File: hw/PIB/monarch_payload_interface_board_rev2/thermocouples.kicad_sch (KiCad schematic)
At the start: 30 parts, among them U3 MAX31856MUD_T, U5 MAX31856MUD_T, U6 MAX31856MUD_T, U7 MAX31856MUD_T, U8 MAX31856MUD_T

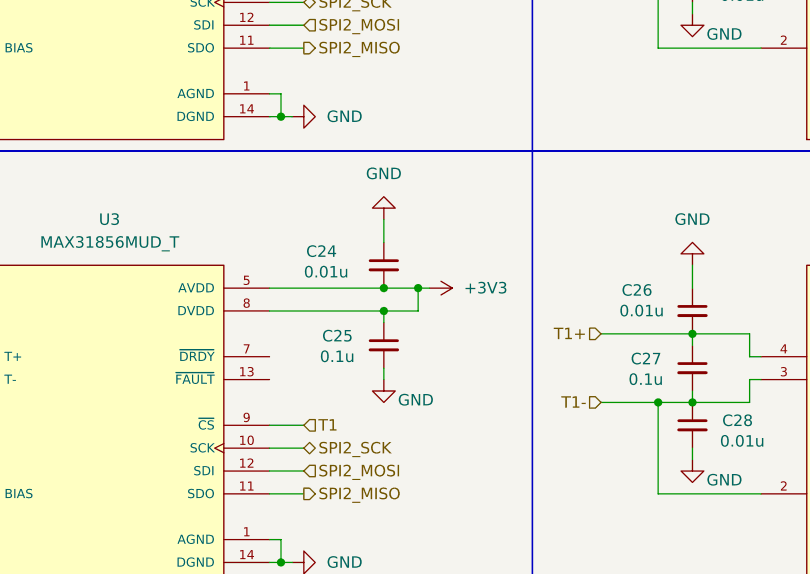
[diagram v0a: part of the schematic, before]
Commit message: AD7124 Fixes
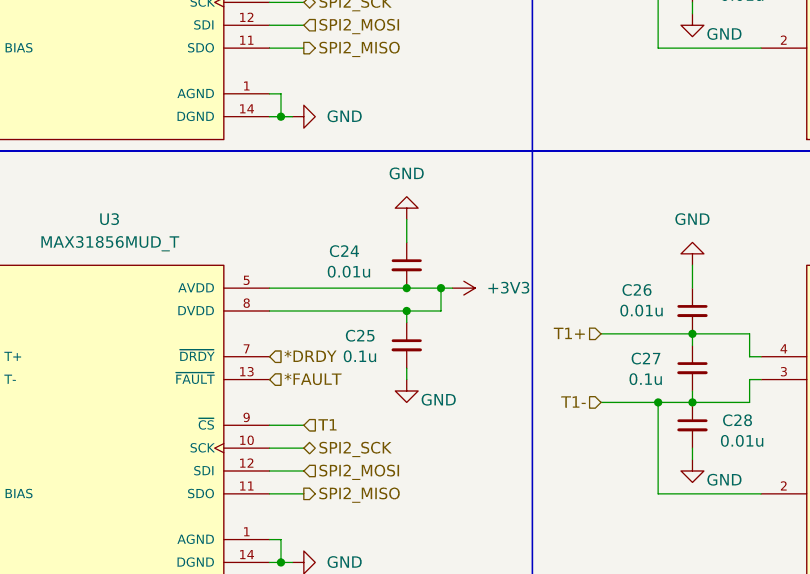
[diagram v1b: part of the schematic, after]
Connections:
- net *FAULT: now reaches U3.13 (~{FAULT})
- net *DRDY: now reaches U3.7 (~{DRDY})
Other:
- moved on the sheet: C24, C25
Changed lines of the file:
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@@
 	)
 	(junction
-		(at 86.36 78.74)
-		(diameter 0)
-		(color 0 0 0 0)
-	)
-	(junction
-		(at 86.36 81.28)
+		(at 88.9 81.28)
 		(diameter 0)
 		(color 0 0 0 0)
@@
 	)
 	(junction
-		(at 90.17 78.74)
+		(at 92.71 78.74)
 		(diameter 0)
 		(color 0 0 0 0)
@@
 	)
 	(junction
+		(at 88.9 78.74)
+		(diameter 0)
+		(color 0 0 0 0)
+	)
+	(junction
 		(at 210.82 34.29)
 		(diameter 0)
@@
 	(wire
 		(pts
-			(xy 86.36 82.55) (xy 86.36 81.28)
+			(xy 88.9 82.55) (xy 88.9 81.28)
 		)
 		(stroke
@@
 	(wire
 		(pts
-			(xy 90.17 78.74) (xy 91.44 78.74)
-		)
-		(stroke
-			(width 0)
-			(type default)
-		)
-	)
-	(wire
-		(pts
 			(xy 128.27 88.9) (xy 127 88.9)
 		)
@@
 	(wire
 		(pts
+			(xy 73.66 78.74) (xy 88.9 78.74)
+		)
+		(stroke
+			(width 0)
+			(type default)
+		)
+	)
+	(wire
+		(pts
 			(xy 110.49 41.91) (xy 116.84 41.91)
 		)
@@
 	(wire
 		(pts
-			(xy 86.36 88.9) (xy 86.36 87.63)
+			(xy 88.9 88.9) (xy 88.9 87.63)
 		)
 		(stroke
@@
 	(wire
 		(pts
-			(xy 73.66 78.74) (xy 86.36 78.74)
+			(xy 38.1 36.83) (xy 36.83 36.83)
 		)
 		(stroke
@@
 	(wire
 		(pts
-			(xy 38.1 36.83) (xy 36.83 36.83)
+			(xy 73.66 96.52) (xy 77.47 96.52)
 		)
 		(stroke
@@
 	(wire
 		(pts
-			(xy 73.66 96.52) (xy 77.47 96.52)
+			(xy 38.1 39.37) (xy 36.83 39.37)
 		)
 		(stroke
@@
 	(wire
 		(pts
-			(xy 38.1 39.37) (xy 36.83 39.37)
+			(xy 207.01 52.07) (xy 207.01 41.91)
 		)
 		(stroke
@@
 	(wire
 		(pts
-			(xy 207.01 52.07) (xy 207.01 41.91)
+			(xy 20.32 91.44) (xy 26.67 91.44)
 		)
 		(stroke
@@
 	(wire
 		(pts
-			(xy 20.32 91.44) (xy 26.67 91.44)
+			(xy 128.27 86.36) (xy 127 86.36)
 		)
 		(stroke
@@
 	(wire
 		(pts
-			(xy 128.27 86.36) (xy 127 86.36)
+			(xy 73.66 81.28) (xy 88.9 81.28)
 		)
 		(stroke
@@
 	(wire
 		(pts
-			(xy 86.36 71.12) (xy 86.36 73.66)
+			(xy 88.9 71.12) (xy 88.9 73.66)
 		)
 		(stroke
@@
 	(wire
 		(pts
-			(xy 90.17 78.74) (xy 90.17 81.28)
+			(xy 92.71 78.74) (xy 92.71 81.28)
 		)
 		(stroke
@@
 	(wire
 		(pts
-			(xy 73.66 81.28) (xy 86.36 81.28)
-		)
-		(stroke
-			(width 0)
-			(type default)
-		)
-	)
-	(wire
-		(pts
-			(xy 86.36 78.74) (xy 90.17 78.74)
+			(xy 88.9 78.74) (xy 93.98 78.74)
 		)
 		(stroke
@@
 	(wire
 		(pts
-			(xy 90.17 81.28) (xy 86.36 81.28)
+			(xy 92.71 81.28) (xy 88.9 81.28)
 		)
 		(stroke
@@
 		)
 	)
+	(hierarchical_label "*FAULT"
+		(shape input)
+		(at 73.66 88.9 0)
+		(effects
+			(font
+				(size 1.27 1.27)
+			)
+			(justify left)
+		)
+	)
 	(hierarchical_label "SPI2_MOSI"
 		(shape input)
@@
 		)
 	)
+	(hierarchical_label "*DRDY"
+		(shape input)
+		(at 73.66 86.36 0)
+		(effects
+			(font
+				(size 1.27 1.27)
+			)
+			(justify left)
+		)
+	)
 	(symbol
 		(lib_id "power:GND")
@@
 	(symbol
 		(lib_id "power:GND")
-		(at 86.36 71.12 180)
+		(at 88.9 71.12 180)
 		(unit 1)
 		(body_style 1)
@@
 		(fields_autoplaced yes)
 		(property "Reference" "#PWR047"
-			(at 86.36 64.77 0)
+			(at 88.9 64.77 0)
 			(hide yes)
 			(show_name no)
@@
 		)
 		(property "Value" "GND"
-			(at 86.36 66.04 0)
+			(at 88.9 66.04 0)
 			(show_name no)
 			(do_not_autoplace no)
@@
 		)
 		(property "Footprint" ""
-			(at 86.36 71.12 0)
+			(at 88.9 71.12 0)
 			(hide yes)
 			(show_name no)
@@
 		)
 		(property "Datasheet" ""
-			(at 86.36 71.12 0)
+			(at 88.9 71.12 0)
 			(hide yes)
 			(show_name no)
@@
 		)
 		(property "Description" "Power symbol creates a global label with name \"GND\" , ground"
-			(at 86.36 71.12 0)
+			(at 88.9 71.12 0)
 			(hide yes)
 			(show_name no)
@@
 	(symbol
 		(lib_id "Device:C_Small")
-		(at 86.36 85.09 0)
+		(at 88.9 85.09 0)
 		(unit 1)
 		(body_style 1)
@@
 		(dnp no)
 		(property "Reference" "C25"
-			(at 79.502 84.074 0)
+			(at 82.042 84.074 0)
 			(show_name no)
 			(do_not_autoplace no)
@@
 		)
 		(property "Value" "0.1u"
-			(at 79.248 86.36 0)
+			(at 81.788 86.36 0)
 			(show_name no)
 			(do_not_autoplace no)
@@
 		)
 		(property "Footprint" "Capacitor_SMD:C_0603_1608Metric"
-			(at 86.36 85.09 0)
+			(at 88.9 85.09 0)
 			(hide yes)
 			(show_name no)
@@
 		)
 		(property "Datasheet" ""
-			(at 86.36 85.09 0)
+			(at 88.9 85.09 0)
 			(hide yes)
 			(show_name no)
@@
 		)
 		(property "Description" "Unpolarized capacitor, small symbol"
-			(at 86.36 85.09 0)
+			(at 88.9 85.09 0)
 			(hide yes)
 			(show_name no)
@@
 	(symbol
 		(lib_id "power:GND")
-		(at 86.36 88.9 0)
+		(at 88.9 88.9 0)
 		(unit 1)
 		(body_style 1)
@@
 		(dnp no)
 		(property "Reference" "#PWR048"
-			(at 86.36 95.25 0)
+			(at 88.9 95.25 0)
 			(hide yes)
 			(show_name no)
@@
 		)
 		(property "Value" "GND"
-			(at 89.916 91.186 0)
+			(at 92.456 91.186 0)
 			(show_name no)
 			(do_not_autoplace no)
@@
 		)
 		(property "Footprint" ""
-			(at 86.36 88.9 0)
+			(at 88.9 88.9 0)
 			(hide yes)
 			(show_name no)
@@
 		)
 		(property "Datasheet" ""
-			(at 86.36 88.9 0)
+			(at 88.9 88.9 0)
 			(hide yes)
 			(show_name no)
@@
 		)
 		(property "Description" "Power symbol creates a global label with name \"GND\" , ground"
-			(at 86.36 88.9 0)
+			(at 88.9 88.9 0)
 			(hide yes)
 			(show_name no)
@@
 	(symbol
 		(lib_id "power:+3V3")
-		(at 91.44 78.74 270)
+		(at 93.98 78.74 270)
 		(unit 1)
 		(body_style 1)
@@
 		(fields_autoplaced yes)
 		(property "Reference" "#PWR046"
-			(at 87.63 78.74 0)
+			(at 90.17 78.74 0)
 			(hide yes)
 			(show_name no)
@@
 		)
 		(property "Value" "+3V3"
-			(at 95.25 78.7399 90)
+			(at 97.79 78.7399 90)
 			(show_name no)
 			(do_not_autoplace no)
@@
 		)
 		(property "Footprint" ""
-			(at 91.44 78.74 0)
+			(at 93.98 78.74 0)
 			(hide yes)
 			(show_name no)
@@
 		)
 		(property "Datasheet" ""
-			(at 91.44 78.74 0)
+			(at 93.98 78.74 0)
 			(hide yes)
 			(show_name no)
@@
 		)
 		(property "Description" "Power symbol creates a global label with name \"+3V3\""
-			(at 91.44 78.74 0)
+			(at 93.98 78.74 0)
 			(hide yes)
 			(show_name no)
@@
 	(symbol
 		(lib_id "Device:C_Small")
-		(at 86.36 76.2 0)
+		(at 88.9 76.2 0)
 		(unit 1)
 		(body_style 1)
@@
 		(dnp no)
 		(property "Reference" "C24"
-			(at 77.724 74.676 0)
+			(at 80.264 74.676 0)
 			(show_name no)
 			(do_not_autoplace no)
@@
 		)
 		(property "Value" "0.01u"
-			(at 77.47 76.962 0)
+			(at 80.01 76.962 0)
 			(show_name no)
 			(do_not_autoplace no)
@@
 		)
 		(property "Footprint" "Capacitor_SMD:C_0603_1608Metric"
-			(at 86.36 76.2 0)
+			(at 88.9 76.2 0)
 			(hide yes)
 			(show_name no)
@@
 		)
 		(property "Datasheet" ""
-			(at 86.36 76.2 0)
+			(at 88.9 76.2 0)
 			(hide yes)
 			(show_name no)
@@
 		)
 		(property "Description" "Unpolarized capacitor, small symbol"
-			(at 86.36 76.2 0)
+			(at 88.9 76.2 0)
 			(hide yes)
 			(show_name no)
